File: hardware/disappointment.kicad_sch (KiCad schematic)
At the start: 62 parts, among them J1 Bus_ISA_16bit, J2 Conn_01x02_Pin, J3 Conn_02x10_Odd_Even, J5 ATX-24, U1 F85226AF, U2 L7905

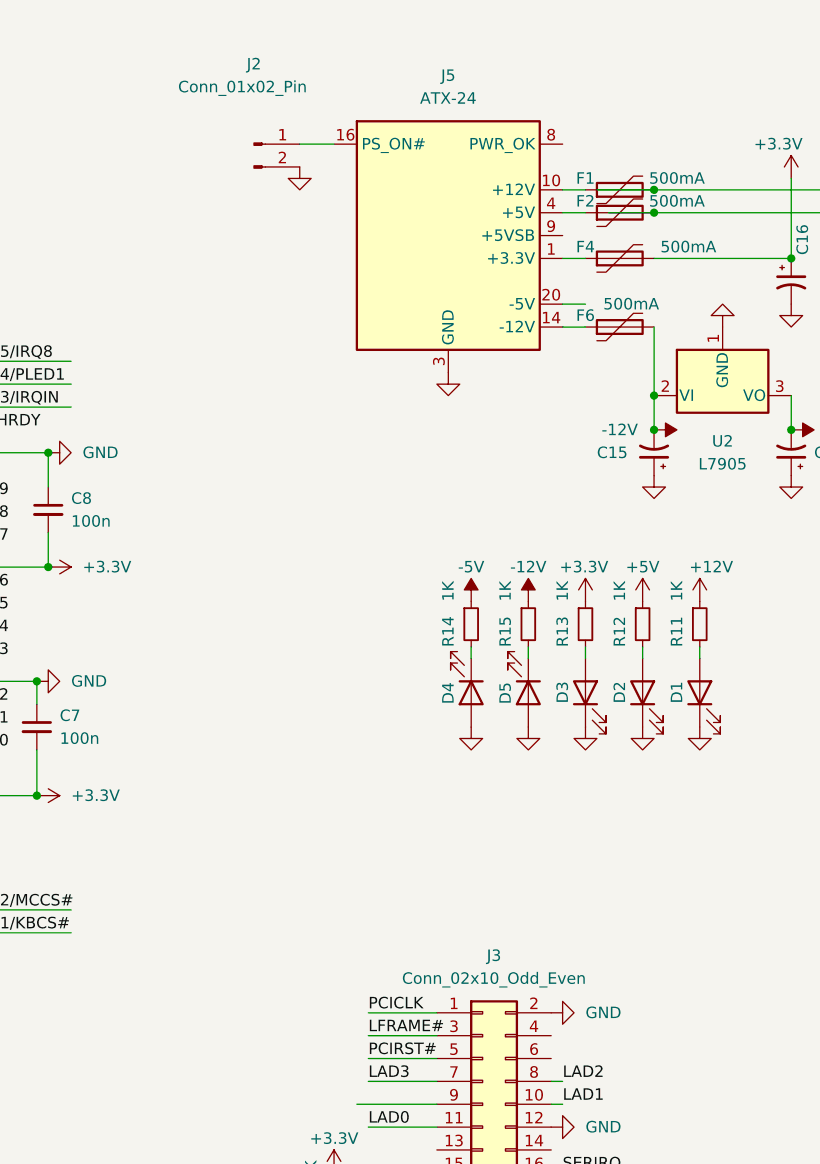
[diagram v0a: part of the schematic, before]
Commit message: what a... letdown?
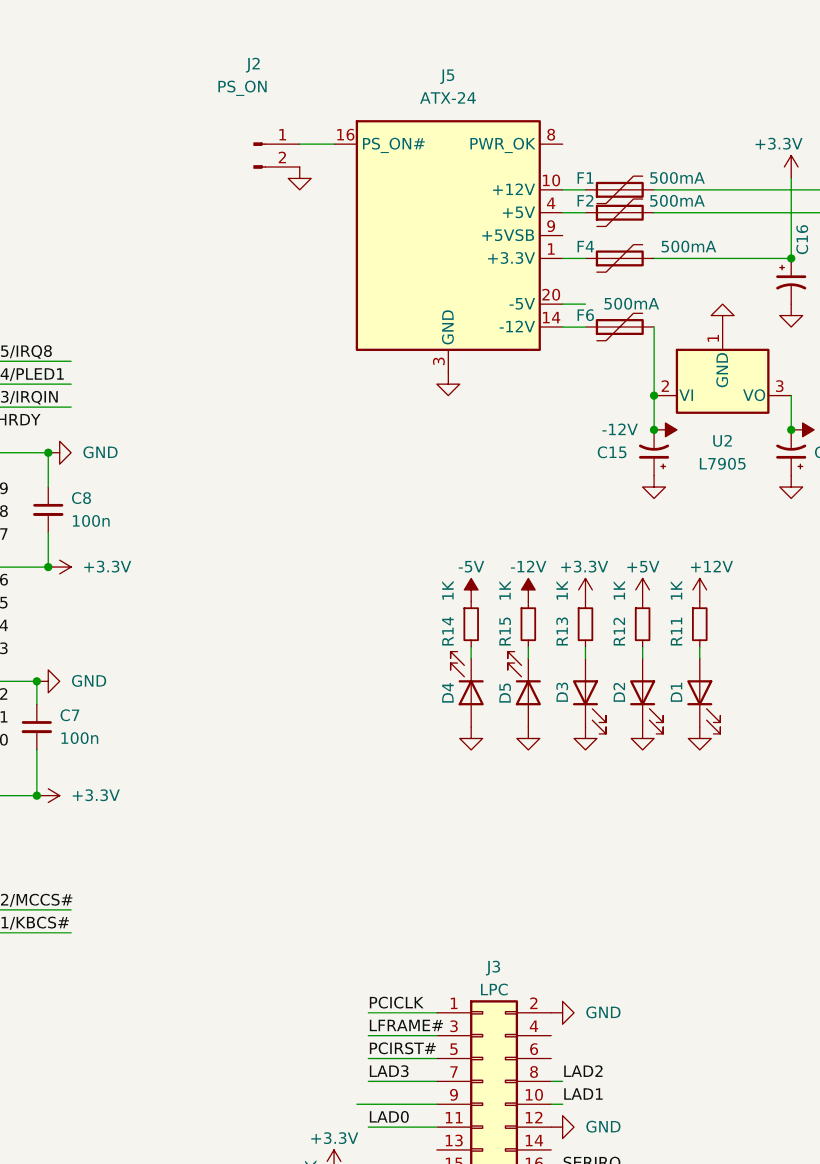
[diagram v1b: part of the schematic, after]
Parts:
- J2: value Conn_01x02_Pin -> PS_ON
- J3: value Conn_02x10_Odd_Even -> LPC
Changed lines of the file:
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@@
   (junction (at 396.24 167.64) (diameter 0) (color 0 0 0 0)
   )
-  (junction (at 345.44 149.86) (diameter 0) (color 0 0 0 0)
-  )
   (junction (at 481.33 193.04) (diameter 0) (color 0 0 0 0)
   )
   (junction (at 124.46 224.79) (diameter 0) (color 0 0 0 0)
   )
-  (junction (at 345.44 152.4) (diameter 0) (color 0 0 0 0)
-  )
   (junction (at 124.46 186.69) (diameter 0) (color 0 0 0 0)
   )
@@
     (stroke (width 0) (type default))
   )
-  (wire (pts (xy 340.36 152.4) (xy 345.44 152.4))
-    (stroke (width 0) (type default))
-  )
   (wire (pts (xy 416.56 139.7) (xy 425.45 139.7))
     (stroke (width 0) (type default))
@@
     (stroke (width 0) (type default))
   )
-  (wire (pts (xy 339.09 149.86) (xy 345.44 149.86))
-    (stroke (width 0) (type default))
-  )
   (label "IRQ7" (at 425.45 190.5 180) (fields_autoplaced)
     (effects (font (size 1.27 1.27)) (justify right bottom))
@@
       (effects (font (size 1.27 1.27)))
     )
-    (property "Value" "Conn_01x02_Pin" (at 299.72 138.43 0)
+    (property "Value" "PS_ON" (at 299.72 138.43 0)
       (effects (font (size 1.27 1.27)))
     )
@@
   (symbol (lib_id "Connector_Generic:Conn_02x10_Odd_Even") (at 326.39 251.46 0) (unit 1)
     (in_bom yes) (on_board yes) (dnp no) (fields_autoplaced)
-    (property "Reference" "J3" (at 327.66 234.95 0)
+    (property "Reference" "J3" (at 327.66 236.22 0)
       (effects (font (size 1.27 1.27)))
     )
-    (property "Value" "Conn_02x10_Odd_Even" (at 327.66 237.49 0)
+    (property "Value" "LPC" (at 327.66 238.76 0)
       (effects (font (size 1.27 1.27)))
     )
